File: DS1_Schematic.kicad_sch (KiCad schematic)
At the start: 58 parts, among them J1 AudioJack3_Switch, J2 AudioJack2_Switch, J3 BAT_CON, J4 PWR_SUPP_COM, Q1 2SC2240, Q2 2SC2240, Q3 2SC2240, U1 NE5532

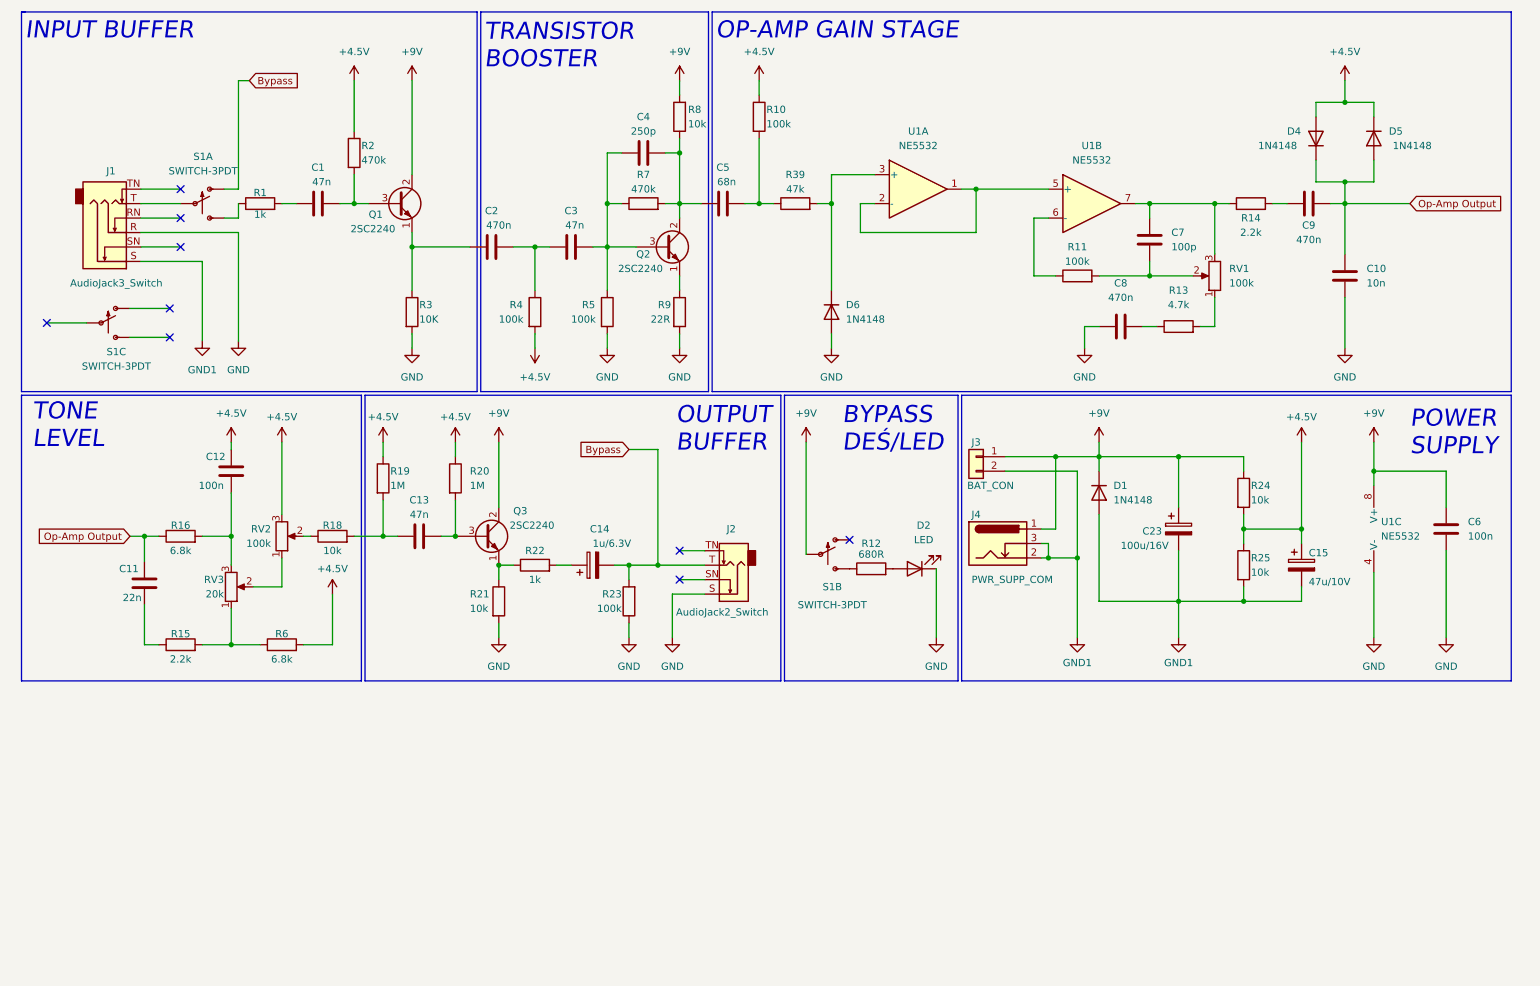
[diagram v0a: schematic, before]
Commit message: version 2.2.1
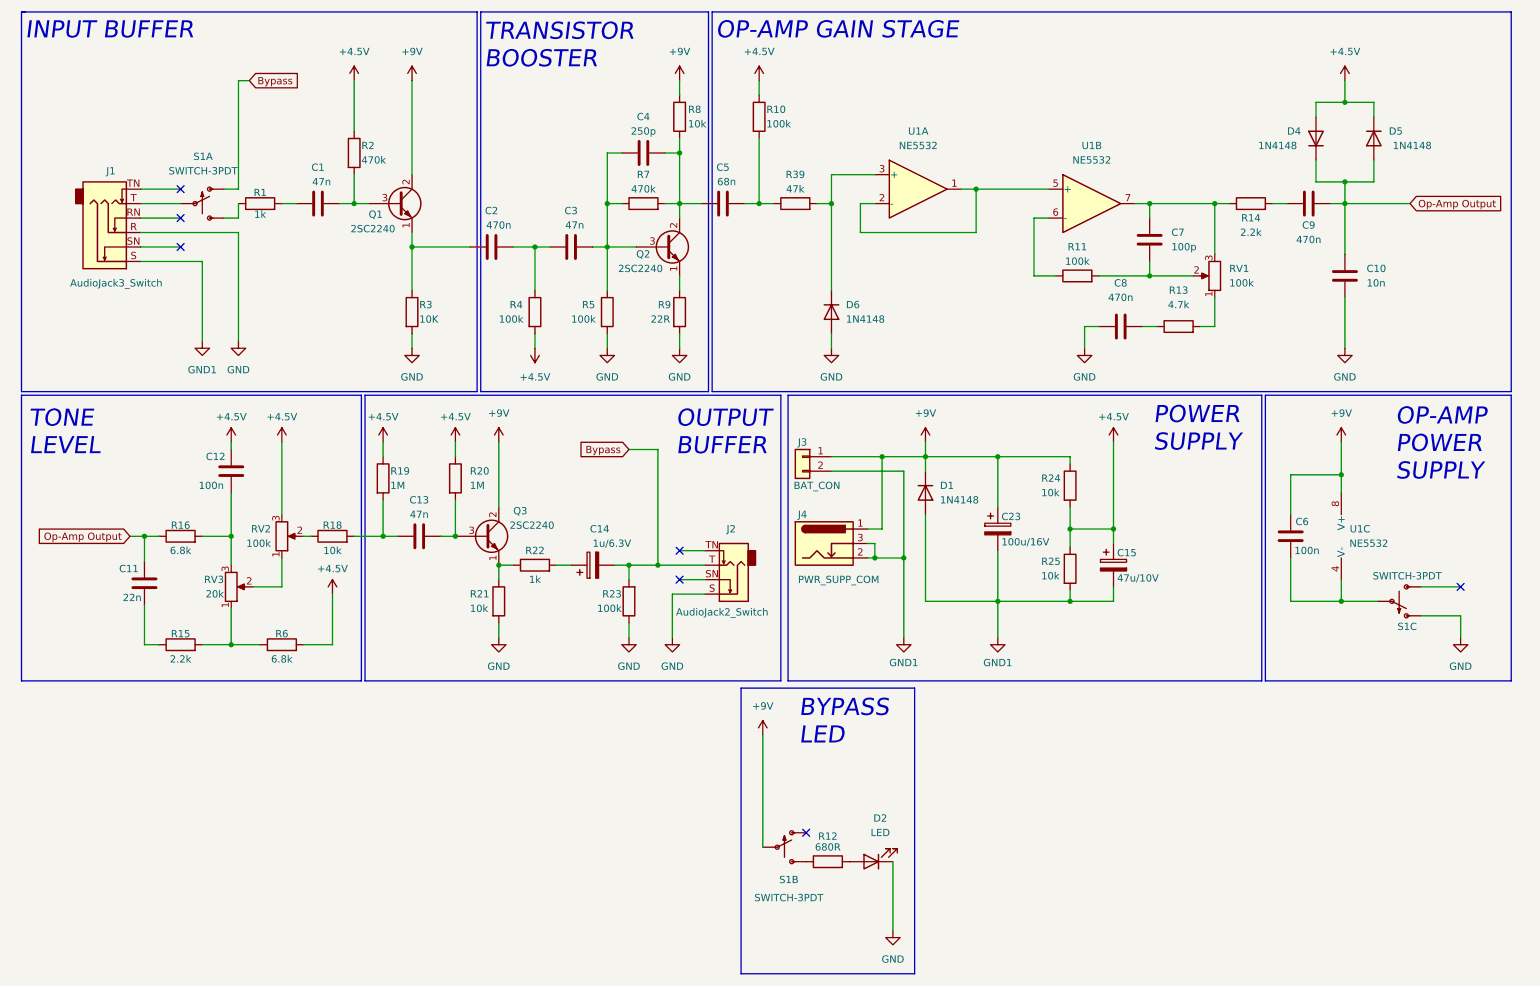
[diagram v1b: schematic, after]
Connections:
- net GND: now also S1.P$7 (O); no longer C6.2, U1.4 (V-)
- net at S1.P$8 (P): now also C6.2, U1.4 (V-)
- no-connect marks 9 -> 7
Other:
- note added: "BYPASS LED"
- note added: "OP-AMP POWER SUPPLY"
- note removed: "BYPASS DEŚ/LED"
- moved on the sheet: C15, C23, C6, D1, D2, J3, J4, R12, R24, R25, S1B, S1C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
